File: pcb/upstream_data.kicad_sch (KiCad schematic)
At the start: 11 parts, among them J6 USB-C, U12 USBLC6-2SC6

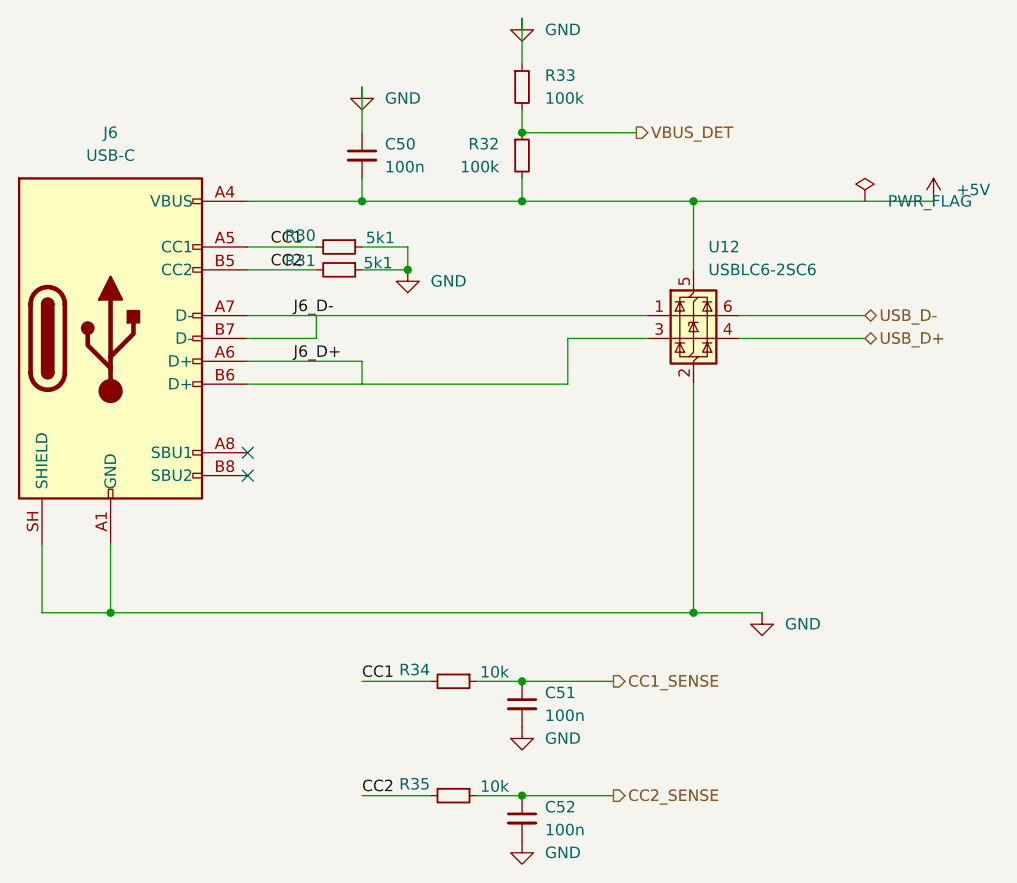
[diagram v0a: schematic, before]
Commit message: manual pcb finishing work
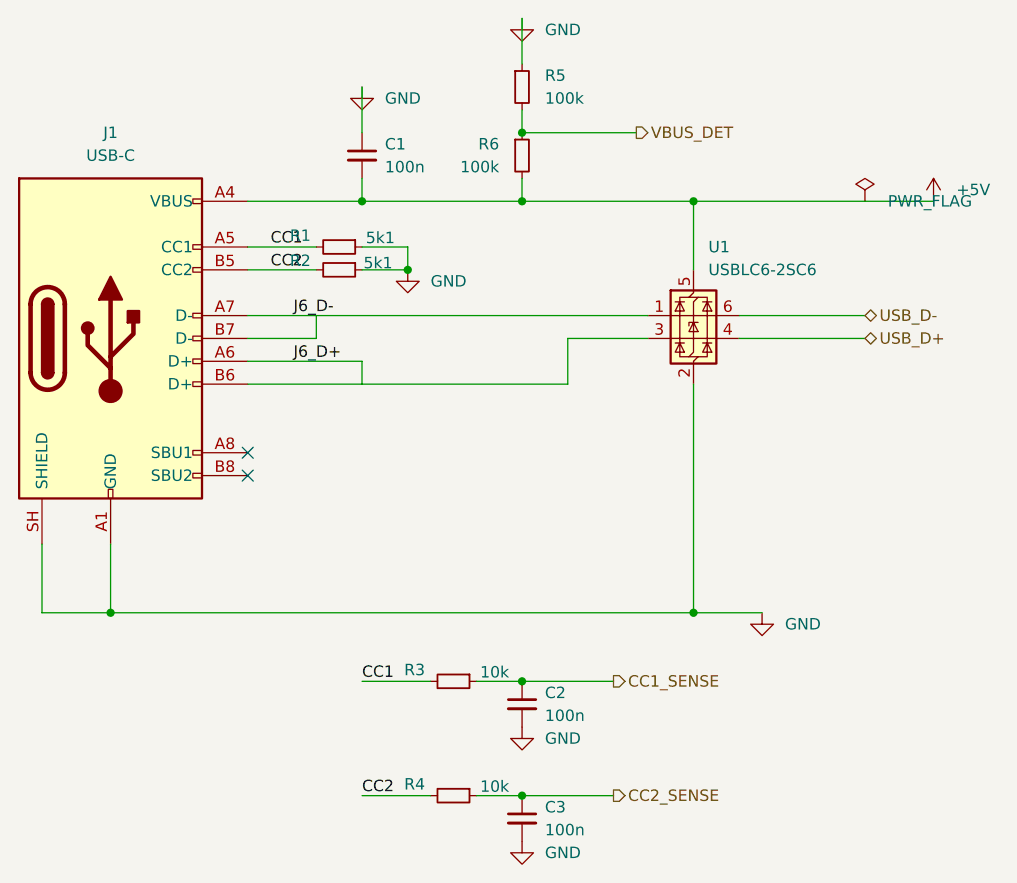
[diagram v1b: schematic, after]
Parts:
- renumbered C50 to C1, C51 to C2, C52 to C3, J6 to J1, R30 to R1, R31 to R2, R34 to R3, R35 to R4, R33 to R5, R32 to R6, U12 to U1
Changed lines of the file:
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@@
 		(dnp no)
 		(fields_autoplaced yes)
-		(property "Reference" "#PWR136"
+		(property "Reference" "#PWR08"
 			(at 121.92 149.86 0)
 			(hide yes)
@@
 			(project "crossfire"
 				(path "/4c5cdd13-4f54-43b0-affb-0ae4b9a4d279/9de577d2-4349-45dc-ab43-167b038179a9"
-					(reference "#PWR136")
+					(reference "#PWR08")
 					(unit 1)
 				)
@@
 		(dnp no)
 		(fields_autoplaced yes)
-		(property "Reference" "#PWR134"
+		(property "Reference" "#PWR011"
 			(at 162.56 96.5199 0)
 			(hide yes)
@@
 			(project "crossfire"
 				(path "/4c5cdd13-4f54-43b0-affb-0ae4b9a4d279/9de577d2-4349-45dc-ab43-167b038179a9"
-					(reference "#PWR134")
+					(reference "#PWR011")
 					(unit 1)
 				)
@@
 		(dnp no)
 		(fields_autoplaced yes)
-		(property "Reference" "R33"
+		(property "Reference" "R5"
 			(at 124.46 85.0899 0)
 			(show_name no)
@@
 			(project "crossfire"
 				(path "/4c5cdd13-4f54-43b0-affb-0ae4b9a4d279/9de577d2-4349-45dc-ab43-167b038179a9"
-					(reference "R33")
+					(reference "R5")
 					(unit 1)
 				)
@@
 		(dnp no)
 		(fields_autoplaced yes)
-		(property "Reference" "C51"
+		(property "Reference" "C2"
 			(at 124.46 153.6762 0)
 			(show_name no)
@@
 			(project "crossfire"
 				(path "/4c5cdd13-4f54-43b0-affb-0ae4b9a4d279/9de577d2-4349-45dc-ab43-167b038179a9"
-					(reference "C51")
+					(reference "C2")
 					(unit 1)
 				)
@@
 		(dnp no)
 		(fields_autoplaced yes)
-		(property "Reference" "#PWR108"
+		(property "Reference" "#PWR05"
 			(at 104.14 78.74 0)
 			(hide yes)
@@
 			(project "crossfire"
 				(path "/4c5cdd13-4f54-43b0-affb-0ae4b9a4d279/9de577d2-4349-45dc-ab43-167b038179a9"
-					(reference "#PWR108")
+					(reference "#PWR05")
 					(unit 1)
 				)
@@
 		(in_pos_files yes)
 		(dnp no)
-		(property "Reference" "R30"
+		(property "Reference" "R1"
 			(at 97.282 102.87 90)
 			(show_name no)
@@
 			(project "crossfire"
 				(path "/4c5cdd13-4f54-43b0-affb-0ae4b9a4d279/9de577d2-4349-45dc-ab43-167b038179a9"
-					(reference "R30")
+					(reference "R1")
 					(unit 1)
 				)
@@
 		(dnp no)
 		(fields_autoplaced yes)
-		(property "Reference" "#PWR135"
+		(property "Reference" "#PWR012"
 			(at 167.64 91.44 0)
 			(hide yes)
@@
 			(project "crossfire"
 				(path "/4c5cdd13-4f54-43b0-affb-0ae4b9a4d279/9de577d2-4349-45dc-ab43-167b038179a9"
-					(reference "#PWR135")
+					(reference "#PWR012")
 					(unit 1)
 				)
@@
 		(in_pos_files yes)
 		(dnp no)
-		(property "Reference" "R31"
+		(property "Reference" "R2"
 			(at 97.282 105.664 90)
 			(show_name no)
@@
 			(project "crossfire"
 				(path "/4c5cdd13-4f54-43b0-affb-0ae4b9a4d279/9de577d2-4349-45dc-ab43-167b038179a9"
-					(reference "R31")
+					(reference "R2")
 					(unit 1)
 				)
@@
 		(in_pos_files yes)
 		(dnp no)
-		(property "Reference" "R35"
+		(property "Reference" "R4"
 			(at 109.982 163.83 90)
 			(show_name no)
@@
 			(project "crossfire"
 				(path "/4c5cdd13-4f54-43b0-affb-0ae4b9a4d279/9de577d2-4349-45dc-ab43-167b038179a9"
-					(reference "R35")
+					(reference "R4")
 					(unit 1)
 				)
@@
 		(dnp no)
 		(fields_autoplaced yes)
-		(property "Reference" "C50"
+		(property "Reference" "C1"
 			(at 106.68 92.7162 0)
 			(show_name no)
@@
 			(project "crossfire"
 				(path "/4c5cdd13-4f54-43b0-affb-0ae4b9a4d279/9de577d2-4349-45dc-ab43-167b038179a9"
-					(reference "C50")
+					(reference "C1")
 					(unit 1)
 				)
@@
 		(dnp no)
 		(fields_autoplaced yes)
-		(property "Reference" "J6"
+		(property "Reference" "J1"
 			(at 76.2 91.44 0)
 			(show_name no)
@@
 			(project "crossfire"
 				(path "/4c5cdd13-4f54-43b0-affb-0ae4b9a4d279/9de577d2-4349-45dc-ab43-167b038179a9"
-					(reference "J6")
+					(reference "J1")
 					(unit 1)
 				)
@@
 		(dnp no)
 		(fields_autoplaced yes)
-		(property "Reference" "C52"
+		(property "Reference" "C3"
 			(at 124.46 166.3762 0)
 			(show_name no)
@@
 			(project "crossfire"
 				(path "/4c5cdd13-4f54-43b0-affb-0ae4b9a4d279/9de577d2-4349-45dc-ab43-167b038179a9"
-					(reference "C52")
+					(reference "C3")
 					(unit 1)
 				)
@@
 		(dnp no)
 		(fields_autoplaced yes)
-		(property "Reference" "#PWR109"
+		(property "Reference" "#PWR06"
 			(at 109.22 99.06 0)
 			(hide yes)
@@
 			(project "crossfire"
 				(path "/4c5cdd13-4f54-43b0-affb-0ae4b9a4d279/9de577d2-4349-45dc-ab43-167b038179a9"
-					(reference "#PWR109")
+					(reference "#PWR06")
 					(unit 1)
 				)
@@
 		(dnp no)
 		(fields_autoplaced yes)
-		(property "Reference" "R32"
+		(property "Reference" "R6"
 			(at 119.38 92.7099 0)
 			(show_name no)
@@
 			(project "crossfire"
 				(path "/4c5cdd13-4f54-43b0-affb-0ae4b9a4d279/9de577d2-4349-45dc-ab43-167b038179a9"
-					(reference "R32")
+					(reference "R6")
 					(unit 1)
 				)
@@
 		(dnp no)
 		(fields_autoplaced yes)
-		(property "Reference" "#PWR137"
+		(property "Reference" "#PWR09"
 			(at 121.92 162.56 0)
 			(hide yes)
@@
 			(project "crossfire"
 				(path "/4c5cdd13-4f54-43b0-affb-0ae4b9a4d279/9de577d2-4349-45dc-ab43-167b038179a9"
-					(reference "#PWR137")
+					(reference "#PWR09")
 					(unit 1)
 				)
@@
 		(dnp no)
 		(fields_autoplaced yes)
-		(property "Reference" "#PWR110"
+		(property "Reference" "#PWR010"
 			(at 148.59 137.16 0)
 			(hide yes)
@@
 			(project "crossfire"
 				(path "/4c5cdd13-4f54-43b0-affb-0ae4b9a4d279/9de577d2-4349-45dc-ab43-167b038179a9"
-					(reference "#PWR110")
+					(reference "#PWR010")
 					(unit 1)
 				)
@@
 		(dnp no)
 		(fields_autoplaced yes)
-		(property "Reference" "U12"
+		(property "Reference" "U1"
 			(at 142.6211 104.14 0)
 			(show_name no)
@@
 			(project "crossfire"
 				(path "/4c5cdd13-4f54-43b0-affb-0ae4b9a4d279/9de577d2-4349-45dc-ab43-167b038179a9"
-					(reference "U12")
+					(reference "U1")
 					(unit 1)
 				)
@@
 		(dnp no)
 		(fields_autoplaced yes)
-		(property "Reference" "#PWR111"
+		(property "Reference" "#PWR07"
 			(at 121.92 71.12 0)
 			(hide yes)
@@
 			(project "crossfire"
 				(path "/4c5cdd13-4f54-43b0-affb-0ae4b9a4d279/9de577d2-4349-45dc-ab43-167b038179a9"
-					(reference "#PWR111")
+					(reference "#PWR07")
 					(unit 1)
 				)
@@
 		(in_pos_files yes)
 		(dnp no)
-		(property "Reference" "R34"
+		(property "Reference" "R3"
 			(at 109.982 151.13 90)
 			(show_name no)
@@
 			(project "crossfire"
 				(path "/4c5cdd13-4f54-43b0-affb-0ae4b9a4d279/9de577d2-4349-45dc-ab43-167b038179a9"
-					(reference "R34")
-					(unit 1)
-				)
+					(reference "R3")
+					(unit 1)
+				)
